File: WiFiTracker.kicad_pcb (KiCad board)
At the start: 2 copper layers, 56.4 x 56.4 mm, 33 parts, among them IC1 CP2104, P1 Battery, P2 USB_B, Q1 MMBT2222A, Q2 MMBT2222A, SW1 SW_RESET, U1 RFM95W-868S2, U2 AP2114, U3 MCP73831T-2ATI/OT, U4 ESP8266-12E

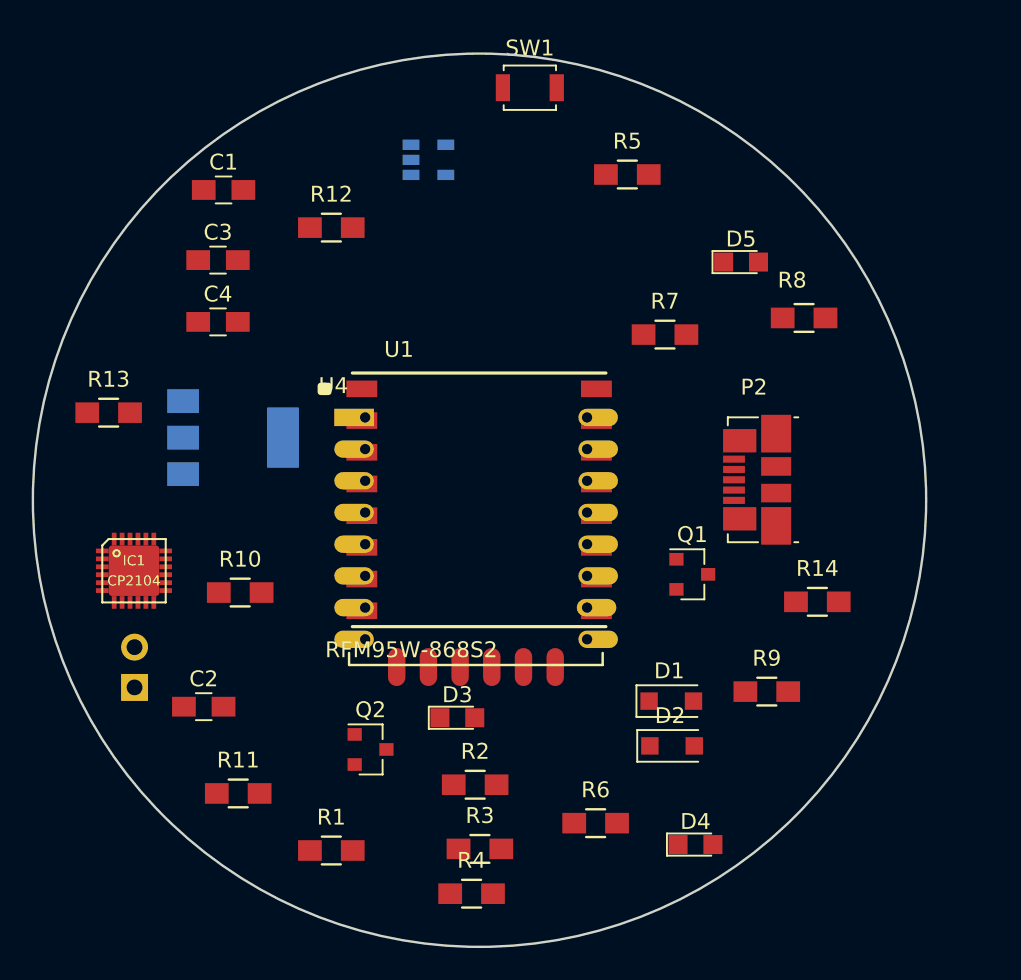
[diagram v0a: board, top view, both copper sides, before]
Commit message: Check PCB V0.1
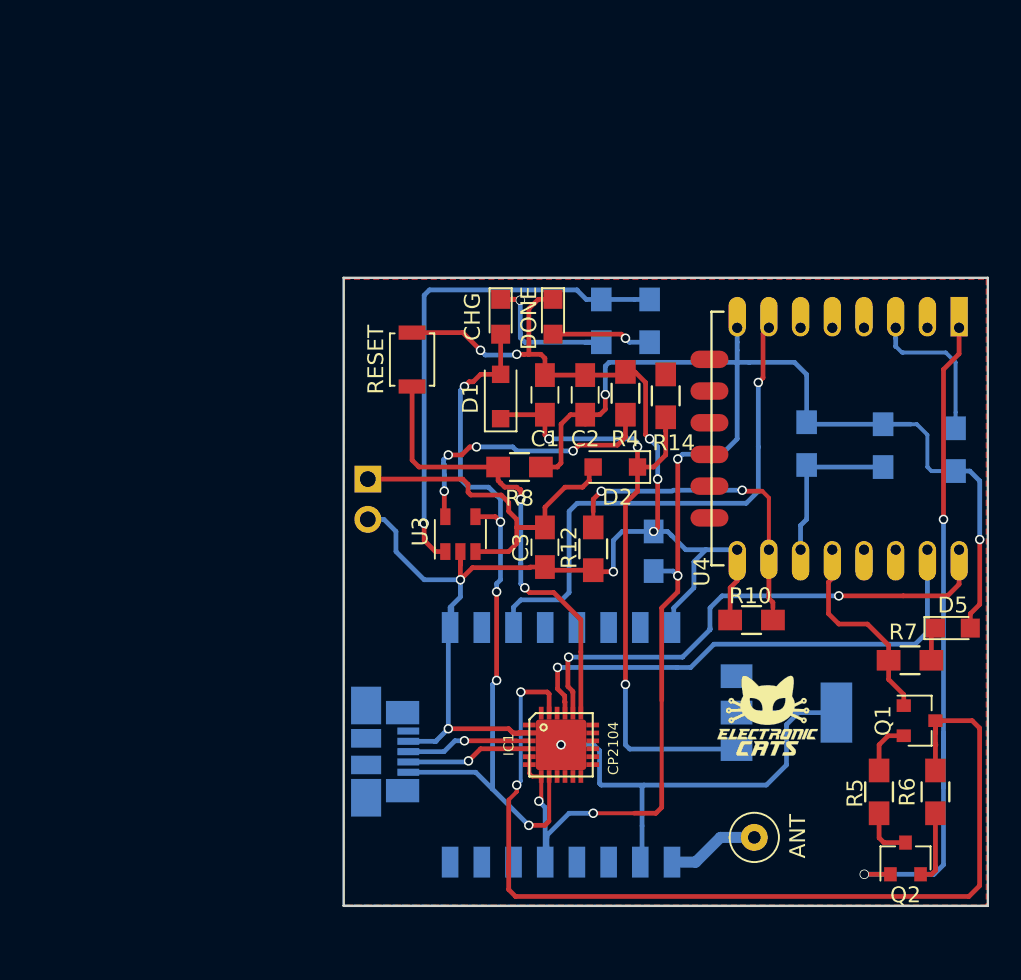
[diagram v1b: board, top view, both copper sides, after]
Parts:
- removed P1: Battery, Pin_Headers:Pin_Header_Angled_1x02_Pitch2.54mm
- removed R3: 10K, Resistors_SMD:R_0805_HandSoldering
- added ANT: ANT, Connect:1pin, F.Cu at (142.7, 110.9)
- added G***: LOGO, TIH:electronic_cats_logo_4x3, F.Cu at (143.5, 103.2)
- added P3: USB_B, Connectors_Molex:USB_Micro-B_Molex_47346-0001, B.Cu at (119.5, 105.5)
- added REF***: OSHW-Logo2_9.8x8mm_SilkScreen, Symbols:OSHW-Logo2_9.8x8mm_SilkScreen, B.Cu at (130.1, 86.2)
- C4, R1, R11, R13, R2: moved to B.Cu
- P2: value USB_B -> Battery; footprint Connectors_Molex:USB_Micro-B_Molex_47346-0001 -> Pin_Headers:Pin_Header_Angled_1x02_Pitch2.54mm; moved to B.Cu
- R4, R8: value 100K -> 10K
- R7: value 100K -> 330R
- R9: value 330R -> 10K; moved to B.Cu
- U1: footprint TIH:XCVR_RFM95W-868S2 -> rfm95:XCVR_RFM95W-868S2; moved to B.Cu
- U3: moved to F.Cu
- moved R13 48.9 mm to (150.8, 86.2), turned to 270 degrees
- moved R11 42.1 mm to (146.0, 86.0), turned to 270 degrees
- moved R5 42.1 mm to (150.5, 108.0), turned to 270 degrees
- moved U2 39.0 mm to (144.7, 103.0)
- moved U4 37.9 mm to (155.6, 78.7), turned to 270 degrees
- moved R1 37.5 mm to (133.0, 78.3), turned to 270 degrees
- moved DONE 34.5 mm to (130.0, 78.0), turned to 270 degrees
- moved Q2 34.4 mm to (152.2, 112.2), turned to 90 degrees
- moved R4 33.0 mm to (134.5, 82.9), turned to 90 degrees
- moved R10 32.3 mm to (142.5, 97.2), turned to 180 degrees
- moved R2 31.3 mm to (136.1, 78.3), turned to 270 degrees
- moved C2 31.1 mm to (132.0, 83.0), turned to 90 degrees
- moved C4 31.1 mm to (136.3, 92.8), turned to 90 degrees
- moved IC1 29.1 mm to (130.5, 105.0)
- moved C3 27.5 mm to (129.5, 92.6), turned to 270 degrees
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- renumbered D3 to CHG, D4 to DONE, SW1 to RESET
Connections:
- P2 pad 1: VCC -> +BATT
- P2 pad 2: Net-(IC1-Pad4) -> GND
- R10 pad 1: +3V3 -> /GPIO15
- R10 pad 2: /RST -> GND
- R11 pad 2: /CH_PD -> /GPIO2
- R4 pad 1: /ADC -> Net-(R4-Pad1)
- R7 pad 1: Net-(R7-Pad1) -> /GPIO0
- R7 pad 2: /ADC -> Net-(D5-Pad1)
- R8 pad 1: /A0 -> +3V3
- R8 pad 2: Net-(R7-Pad1) -> /RST
- R9 pad 1: /GPIO0 -> +3V3
- R9 pad 2: Net-(D5-Pad1) -> /CH_PD
- U1 pad 5: /GPIO15 -> /GPIO16
- U2 pad 3: Net-(R14-Pad1) -> Net-(U2-Pad3)
- U3 pad 5: Net-(R3-Pad1) -> Net-(R4-Pad1)
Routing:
- net GND: track 0.00 -> 128.2 mm, vias 0 -> 9
- net +3V3: track 0.00 -> 102.7 mm, vias 0 -> 6
- net /DTR: track 0.00 -> 63.6 mm, vias 0 -> 2
- net VCC: track 0.00 -> 47.6 mm, vias 0 -> 5
- net /RESET: track 0.00 -> 44.6 mm, vias 0 -> 2
- net Net-(C1-Pad1): track 0.00 -> 41.2 mm, vias 0 -> 3
- net /GPIO13: track 0.00 -> 33.8 mm, vias 0 -> 1
- net /TXD: track 0.00 -> 33.3 mm, vias 0 -> 2
- net /RXD: track 0.00 -> 33.2 mm, vias 0 -> 1
- net Net-(R1-Pad1): track 0.00 -> 31.7 mm, vias 0 -> 1
- net /RST: track 0.00 -> 29.6 mm, vias 0 -> 2
- net +BATT: track 0.00 -> 24.2 mm
- net /GPIO15: track 0.00 -> 21.4 mm, vias 0 -> 2
- net Net-(R4-Pad1): track 0.00 -> 17.4 mm, vias 0 -> 4
- net /GPIO0: track 0.00 -> 13.0 mm
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- added copper zone on B.Cu, net GND
- added copper zone on F.Cu, net GND
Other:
- board size 56.4 x 56.4 mm -> 40.6 x 39.6 mm
- net class Default: trace_width 0.25 -> 0.3; via_drill 0.4 -> 0.5
- net class VCC added: clearance 0.2, trace_width 0.5, via_dia 0.6, via_drill 0.4
- rule trace_min: 0.2 -> 0.25
